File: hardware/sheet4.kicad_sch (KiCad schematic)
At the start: 20 parts, among them J2 B4B-XH-A, J3 B-2100S04P-A110, U2 STM32F072CBT6

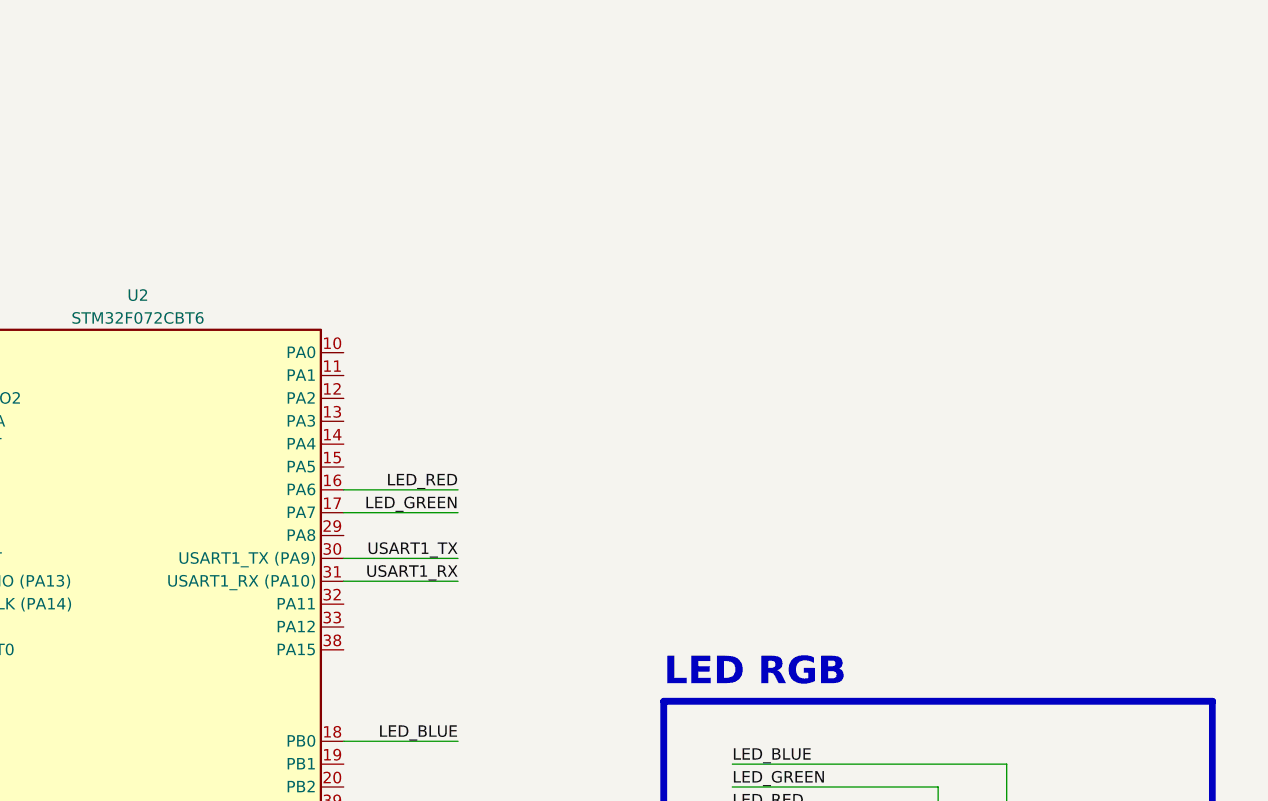
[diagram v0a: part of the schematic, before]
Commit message: hardware(feat): add usb connector with esd (#1)
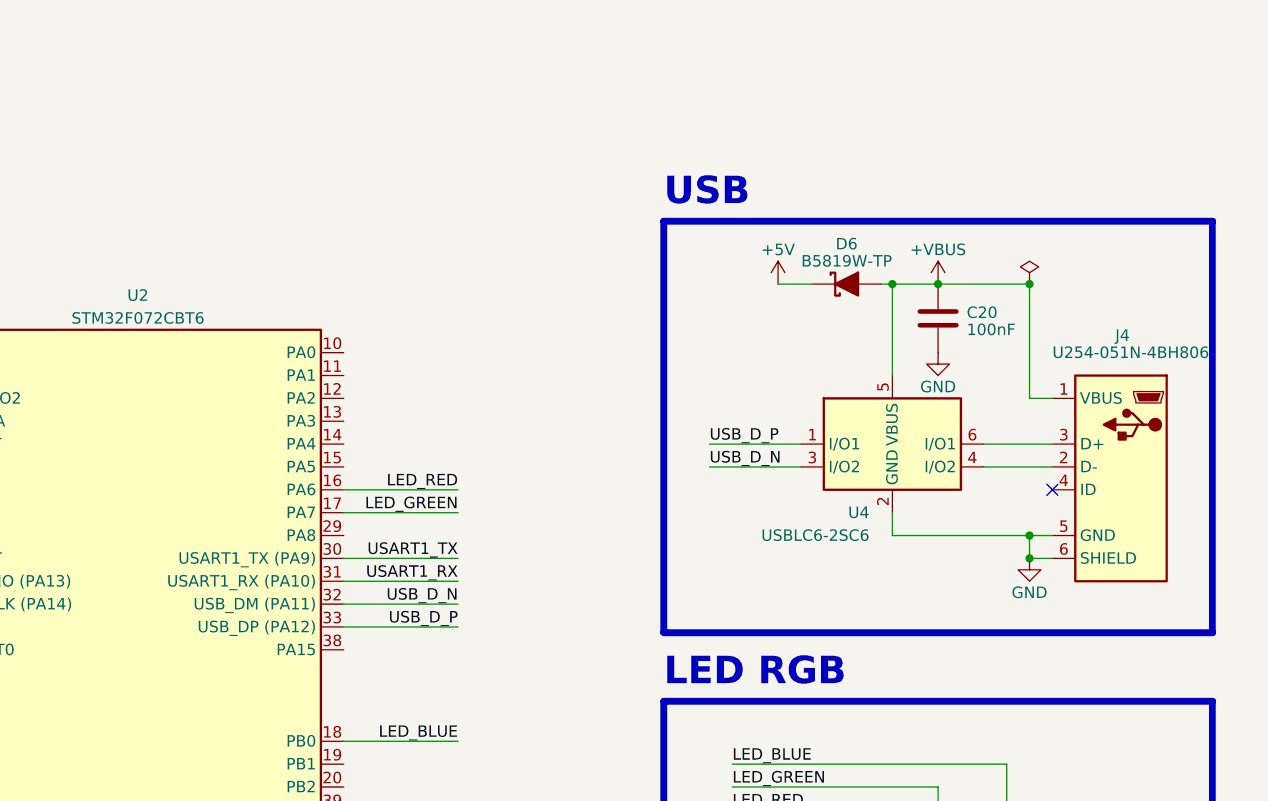
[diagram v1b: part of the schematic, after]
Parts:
- added C20: 100nF, 02_capacitors:C_0603_1608Metric, symbol 02_capacitors:CAP_100nF-50V-10%-X7R-0603
- added D6: B5819W-TP, 04_diodes:D_SOD-123, symbol 04_diodes:DIO-S_40V-1A-0.6V-SOD-123
- added J4: U254-051N-4BH806, 08_connectors:SMD_U254-051N-4BH806, symbol 08_connectors:CON-USB_U254-051N-4BH806
- added U4: USBLC6-2SC6, 06_ics:SOT-23-6, symbol 06_ics:IC-IF_USBLC6-2SC6
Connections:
- net GND: now also C20.2, J4.5 (GND), J4.6 (SHIELD), U4.2 (GND)
- net USB_D_N: now reaches U2.32 (PA11)
- net USB_D_N: now also U4.3 (I/O2)
- net USB_D_P: now reaches U2.33 (PA12)
- net USB_D_P: now also U4.1 (I/O1)
- new net: J4.2 (D-), U4.4 (I/O2)
- new net: J4.3 (D+), U4.6 (I/O1)
- new net +5V: D6.1 (K)
- new net +VBUS: C20.1, D6.2 (A), J4.1 (VBUS), U4.5 (VBUS)
- no-connect marks 0 -> 1
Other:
- note added: "USB"
